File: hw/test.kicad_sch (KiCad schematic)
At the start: 15 parts

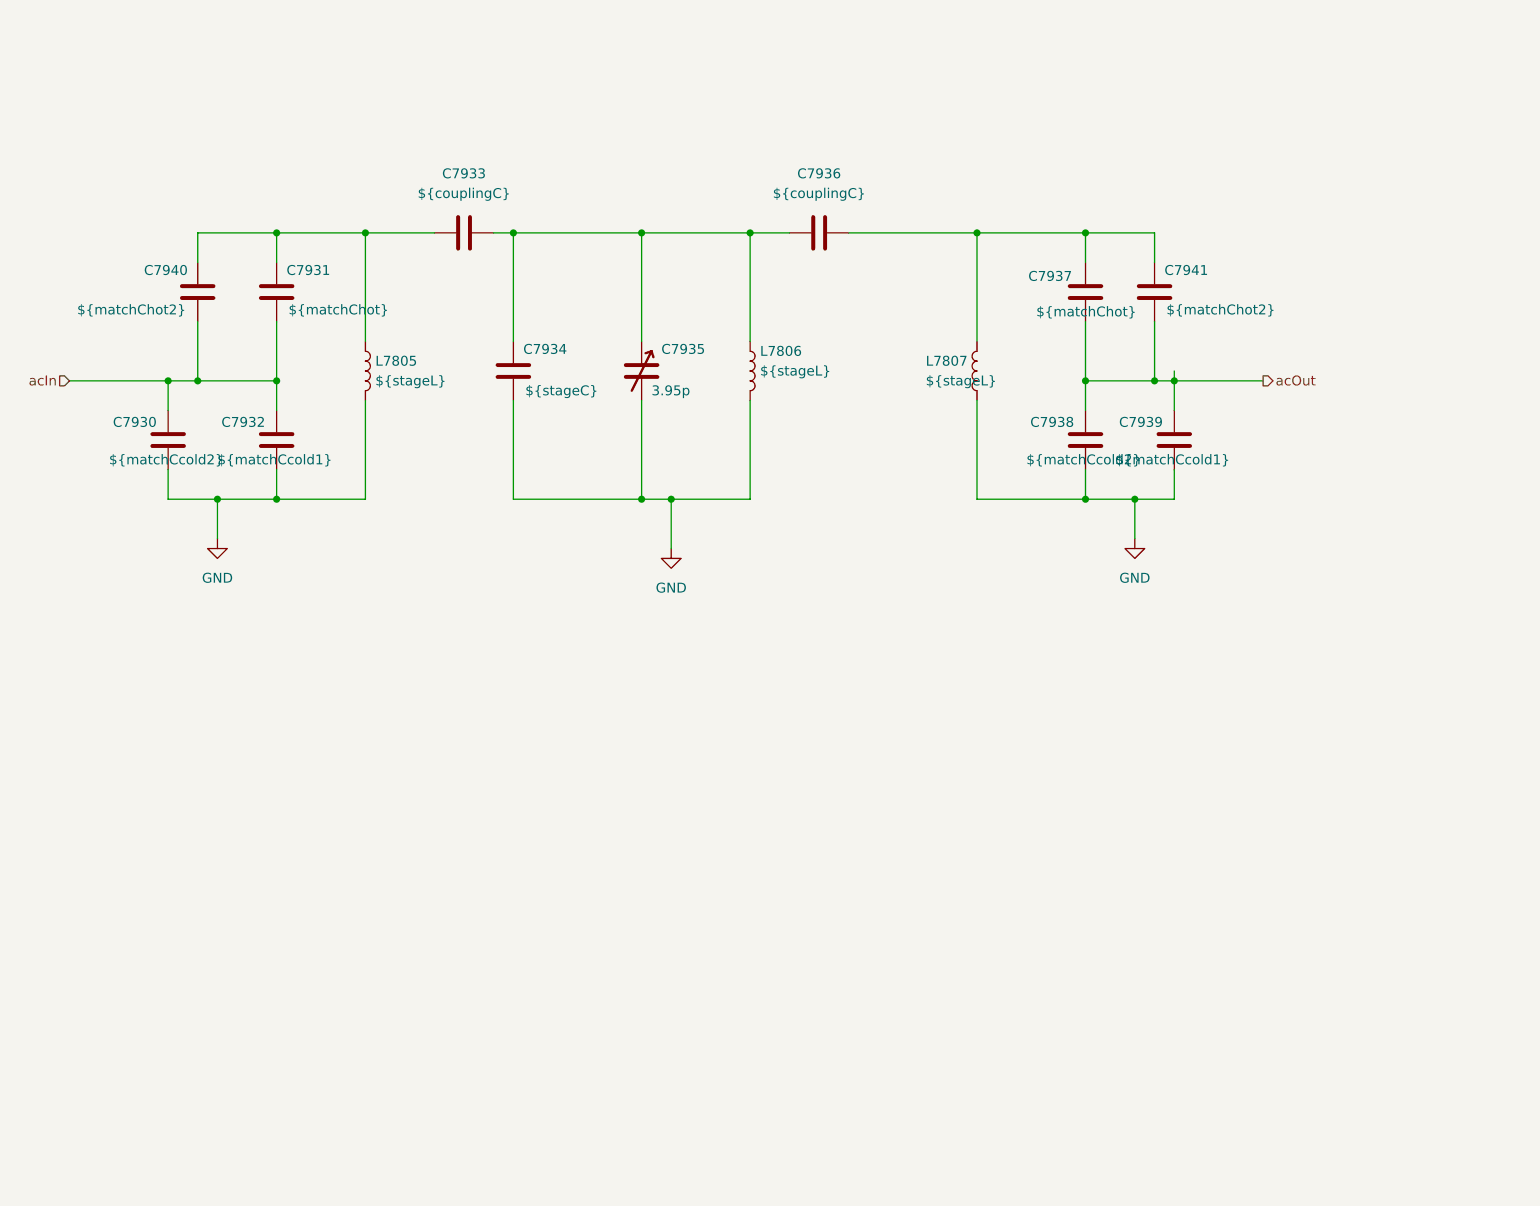
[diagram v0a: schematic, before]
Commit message: Filter calc checkpoint
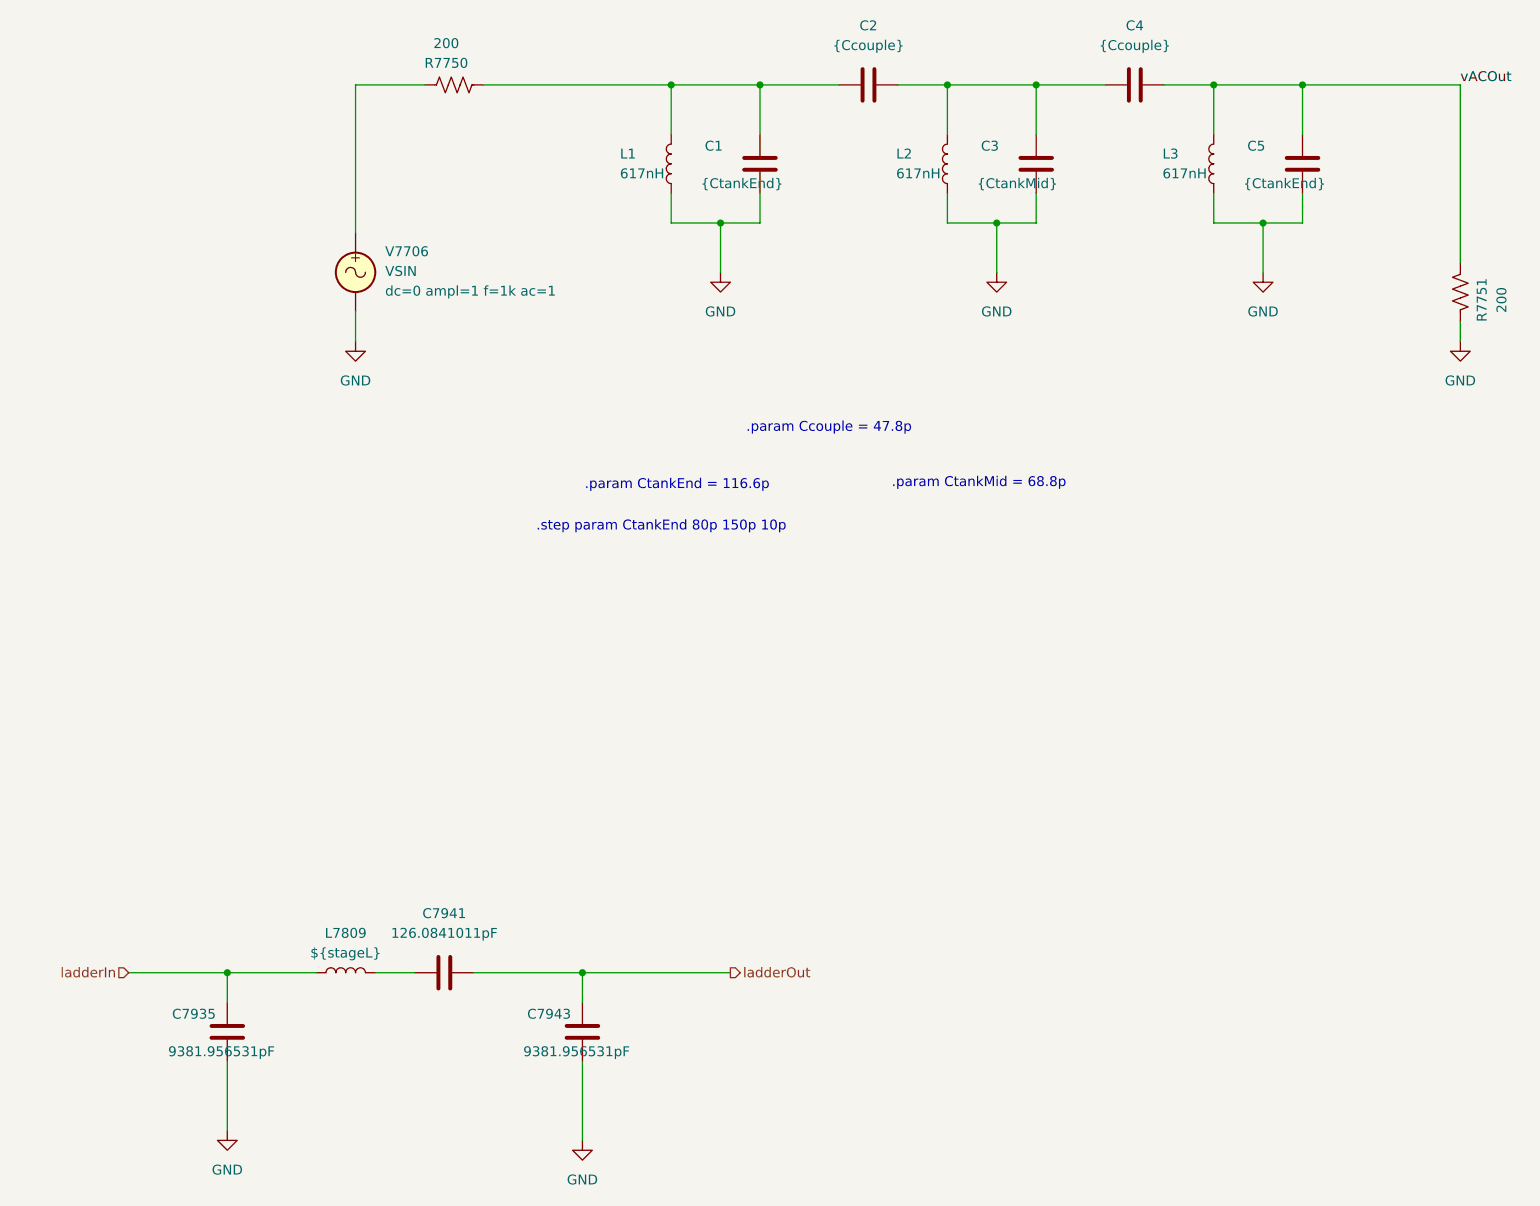
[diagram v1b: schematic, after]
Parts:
- removed C7930: ${matchCcold2}, symbol Device:C
- removed C7931, C7937: ${matchChot}, symbol Device:C
- removed C7932, C7939: ${matchCcold1}, symbol Device:C
- removed C7933: ${couplingC}, symbol Device:C
- removed C7934: ${stageC}, symbol Device:C
- removed C7935: 3.95p, PCM_Capacitor_THT_AKL:C_Trimmer_BFC2-808_L7.3mm_W5.5mm_P5.6mm_Hole, symbol PCM_Capacitor_AKL:C_Trim_Vishay_BFC2-808_D7.5mm_Hole
- removed C7940: ${matchChot2}, symbol Device:C
- removed L7805, L7806: ${stageL}, symbol Device:L
- added C1, C5: {CtankEnd}, symbol Device:C
- added C4: {Ccouple}, symbol Device:C
- added C7935, C7943: 9381.956531pF, symbol Device:C
- added L1, L3: 617nH, symbol Device:L
- added L7809: ${stageL}, symbol Device:L
- added R7750, R7751: 200, symbol Device:R_US
- added V7706: VSIN, symbol Simulation_SPICE:VSIN
- C2: renamed from C7936; value ${couplingC} -> {Ccouple}
- C3: renamed from C7938; value ${matchCcold2} -> {CtankMid}
- C7941: value ${matchChot2} -> 126.0841011pF
- L2: renamed from L7807; value ${stageL} -> 617nH
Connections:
- net GND: now also C1.2, C5.2, C7935.2, C7943.2, L1.2, L3.2, R7751.2, V7706.2
- net at C2.1: now also C1.1, L1.1, R7750.1
- net at C2.2, L2.1: now also C3.1, C4.1; no longer C7941.1
- net acOut renamed ladderOut
- net ladderOut: now also C7943.1; no longer C3.1
- new net: C7941.1, L7809.2
- new net: R7750.2, V7706.1
- new net ladderIn: C7935.1, L7809.1
- new net vACOut: C4.2, C5.1, L3.1, R7751.1
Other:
- note added: ".param Ccouple = 47.8p"
- note added: ".param CtankEnd = 116.6p"
- note added: ".param CtankMid = 68.8p"
- note added: ".step param CtankEnd 80p 150p 10p"
- moved on the sheet: C2, C3, L2
